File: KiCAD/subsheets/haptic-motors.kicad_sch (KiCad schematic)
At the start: 15 parts, among them U3 DRV2605LDGS, U4 DRV2605LDGS

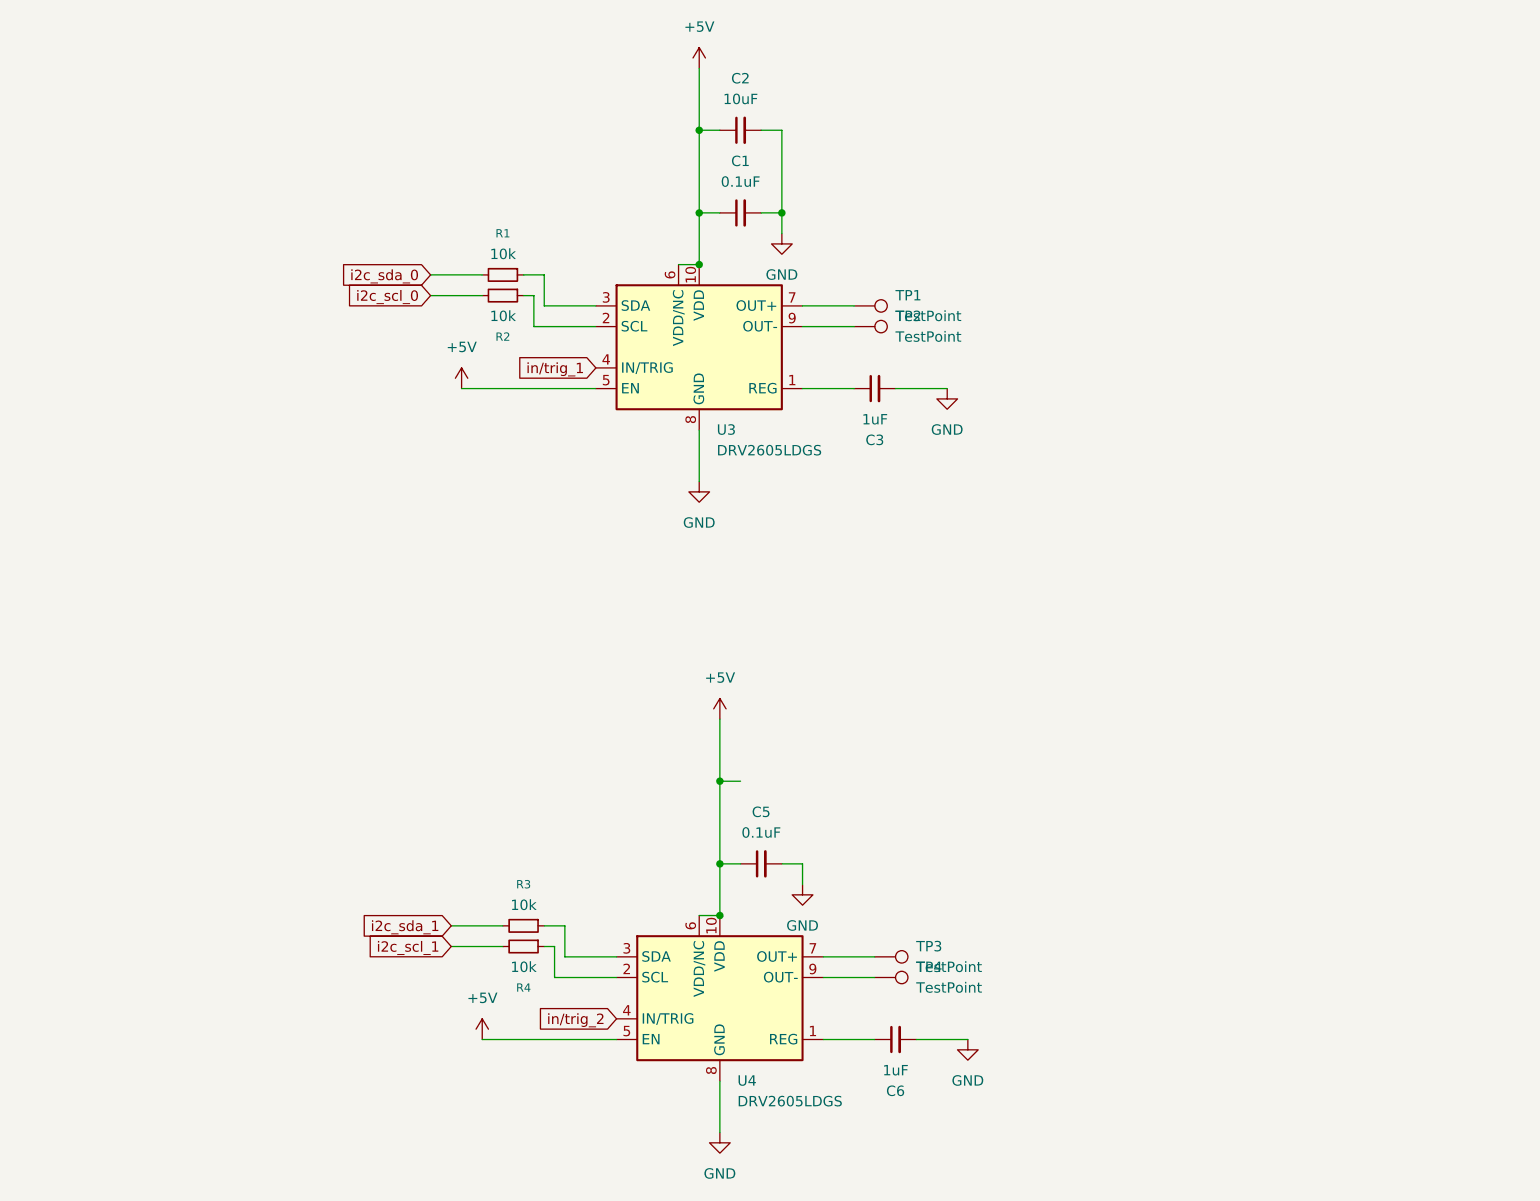
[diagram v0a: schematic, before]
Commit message: schematic
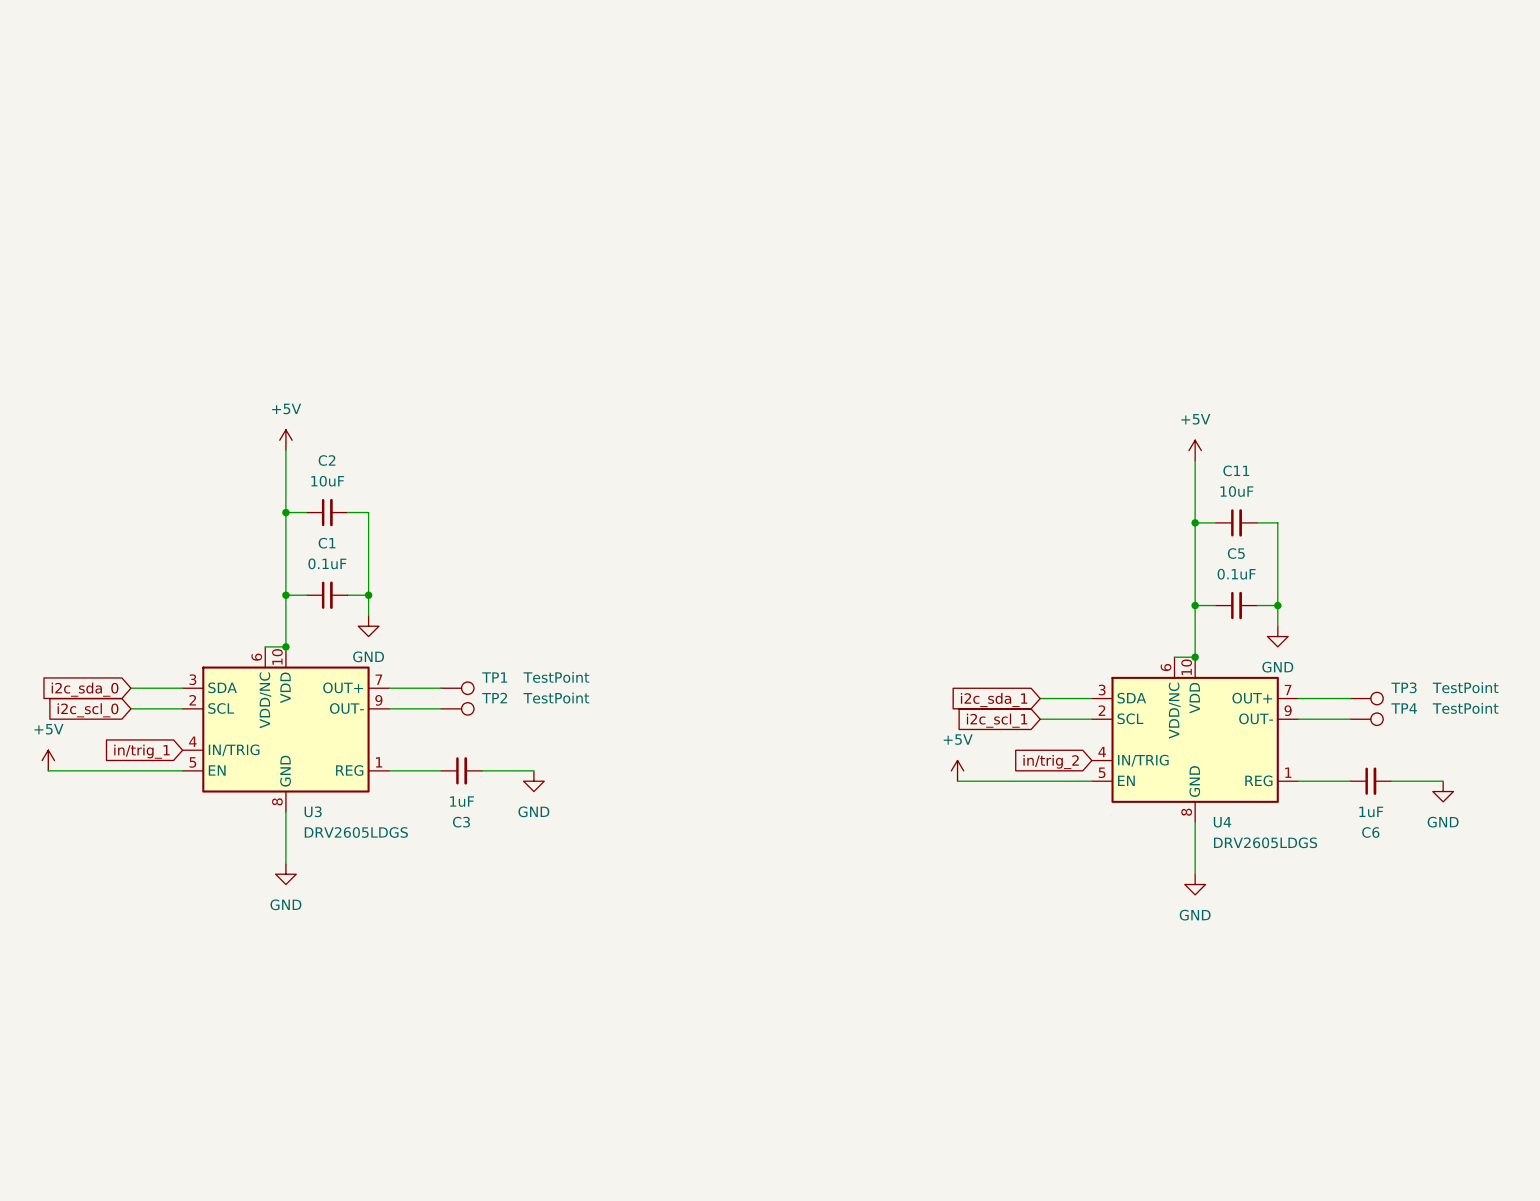
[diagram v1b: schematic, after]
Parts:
- removed R1, R2, R3, R4: 10k, symbol Device:R_Small
- added C11: 10uF, Capacitor_SMD:C_0603_1608Metric, symbol Device:C_Small
- C1, C2, C3, C5, C6: footprint (none) -> Capacitor_SMD:C_0603_1608Metric
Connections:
- net +5V: now also C11.1
- net GND: now also C11.2
- net i2c_scl_0: now also U3.2 (SCL)
- net i2c_scl_1: now also U4.2 (SCL)
- net i2c_sda_0: now also U3.3 (SDA)
- net i2c_sda_1: now also U4.3 (SDA)
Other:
- moved on the sheet: C1, C2, C3, C5, C6, TP1, TP2, TP3, TP4, U3, U4
